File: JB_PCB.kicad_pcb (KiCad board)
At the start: 2 copper layers, 66 x 114.2 mm, 20 parts, among them J1 Conn_01x03_Pin, J10 Conn_01x03_Pin, J12 Conn_01x05_Pin, J2 Screw_Terminal_01x02, J3 Screw_Terminal_01x02, J4 Screw_Terminal_01x02, J5 Conn_01x03_Pin, J6 Screw_Terminal_01x02, J7 Conn_01x03_Pin, J8 Conn_01x03_Pin, J9 Conn_01x03_Pin

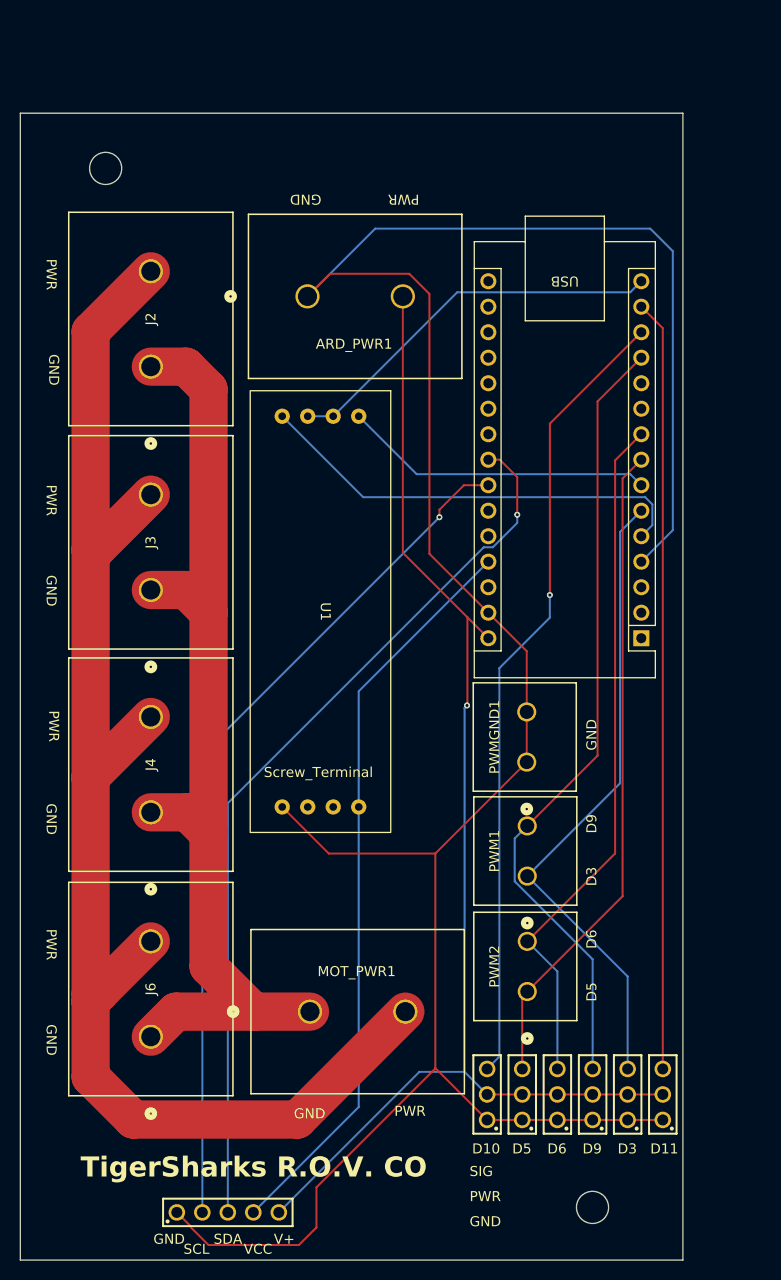
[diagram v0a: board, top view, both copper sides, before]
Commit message: changes from my laptop from last year
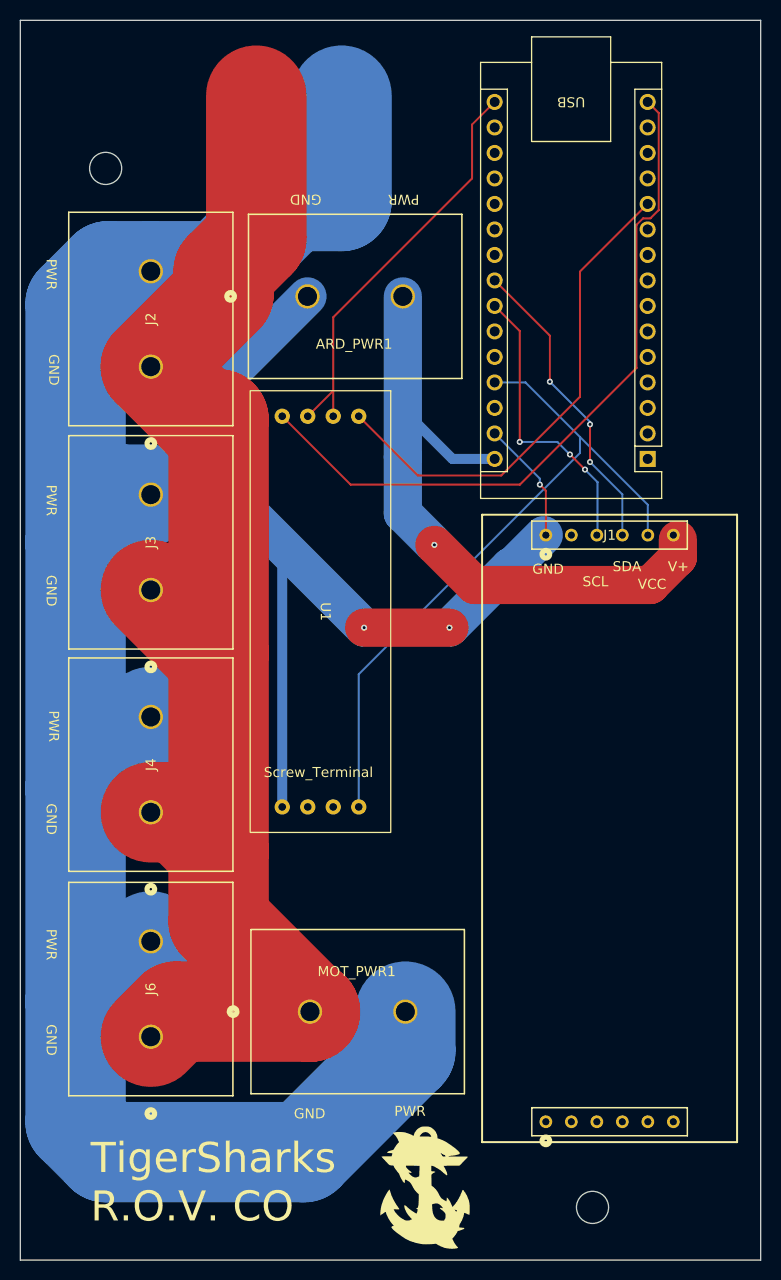
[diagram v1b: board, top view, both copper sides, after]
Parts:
- removed J10, J5, J7, J8, J9: Conn_01x03_Pin, myFootprints.pretty-master:3x1_Pin_Header
- removed J12: Conn_01x05_Pin, myFootprints.pretty-master:1x5conn
- removed PWM1, PWM2, PWMGND1: Screw_Terminal_01x02, myFootprints.pretty-master:screw 2x2
- added G***: LOGO, myFootprints.pretty-master:MateLogo, F.Cu at (142.5, 150.5)
- added REF**: CON6_1X6_TU_HTS_SAI, myFootprints.pretty-master:1x6Headers, F.Cu at (161.2, 144.0)
- J1: value Conn_01x03_Pin -> Conn_01x06_Pin; footprint myFootprints.pretty-master:3x1_Pin_Header -> myFootprints.pretty-master:1x6Headers
- moved J1 57.0 mm to (161.2, 85.5), turned to 0 degrees
- moved A1 17.9 mm to (165.0, 77.9)
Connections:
- A1 pad 11: unconnected-(A1-D8-Pad11) -> Net-(A1-D8)
- A1 pad 12: Net-(A1-D9) -> unconnected-(A1-D9-Pad12)
- A1 pad 13: Net-(A1-D10) -> unconnected-(A1-D10-Pad13)
- A1 pad 14: Net-(A1-D11) -> unconnected-(A1-D11-Pad14)
- A1 pad 16: unconnected-(A1-D13-Pad16) -> Net-(A1-D13)
- A1 pad 27: Net-(A1-+5V) -> Net-(A1-VIN)
- A1 pad 4: Net-(ARD_PWR1-Pin_1) -> unconnected-(A1-GND-Pad4)
- A1 pad 5: Net-(A1-D2) -> unconnected-(A1-D2-Pad5)
- A1 pad 6: Net-(A1-D3) -> unconnected-(A1-D3-Pad6)
- A1 pad 7: Net-(A1-D4) -> unconnected-(A1-D4-Pad7)
- A1 pad 8: Net-(A1-D5) -> unconnected-(A1-D5-Pad8)
- A1 pad 9: Net-(A1-D6) -> unconnected-(A1-D6-Pad9)
- J1 pad 2: Net-(A1-VIN) -> unconnected-(J1-Pin_2-Pad2)
- J1 pad 3: Net-(A1-D10) -> Net-(A1-A5)
- U1 pad DE: Net-(A1-D12) -> Net-(A1-D13)
- U1 pad DI: Net-(A1-D2) -> Net-(A1-D12)
- U1 pad RE: Net-(A1-D12) -> Net-(A1-D13)
- U1 pad RO: Net-(A1-D4) -> Net-(A1-D8)
- U1 pad VCC: Net-(A1-+5V) -> Net-(A1-VIN)
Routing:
- net Net-(ARD_PWR1-Pin_1): track 250.0 -> 102.2 mm, vias 0 -> 3
- net Net-(A1-D10): track 79.8 -> 0.00 mm, vias 1 -> 0
- net Net-(A1-D9): track 79.3 -> 0.00 mm
- net Net-(A1-D11): track 76.8 -> 0.00 mm
- net Net-(A1-+5V): track 74.5 -> 0.00 mm
- net Net-(A1-D6): track 69.2 -> 0.00 mm
- net Net-(A1-D5): track 65.6 -> 0.00 mm
- net Net-(A1-D3): track 64.5 -> 0.00 mm
- net Net-(A1-A4): track 89.3 -> 30.6 mm, vias 1 -> 3
- net Net-(A1-A5): track 85.7 -> 29.3 mm, vias 1 -> 3
- net Net-(A1-D8): track 0.00 -> 49.7 mm
- net Net-(J2-Pin_2): track 145.7 -> 194.8 mm
- net Net-(A1-D2): track 44.1 -> 0.00 mm
- net Net-(A1-D13): track 0.00 -> 41.6 mm
- net Net-(J2-Pin_1): track 100.7 -> 137.7 mm
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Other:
- board size 66 x 114.2 mm -> 73.8 x 123.5 mm
- board text removed: "D10"
- board text removed: "D11"
- board text removed: "D3"
- board text removed: "D5"
- board text removed: "D6"
- board text removed: "D9"
- board text removed: "SIG"
